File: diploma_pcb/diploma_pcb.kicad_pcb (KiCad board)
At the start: 2 copper layers, 50 x 24 mm, 16 parts, among them Q1 2SC3356, Q3 2SC3356

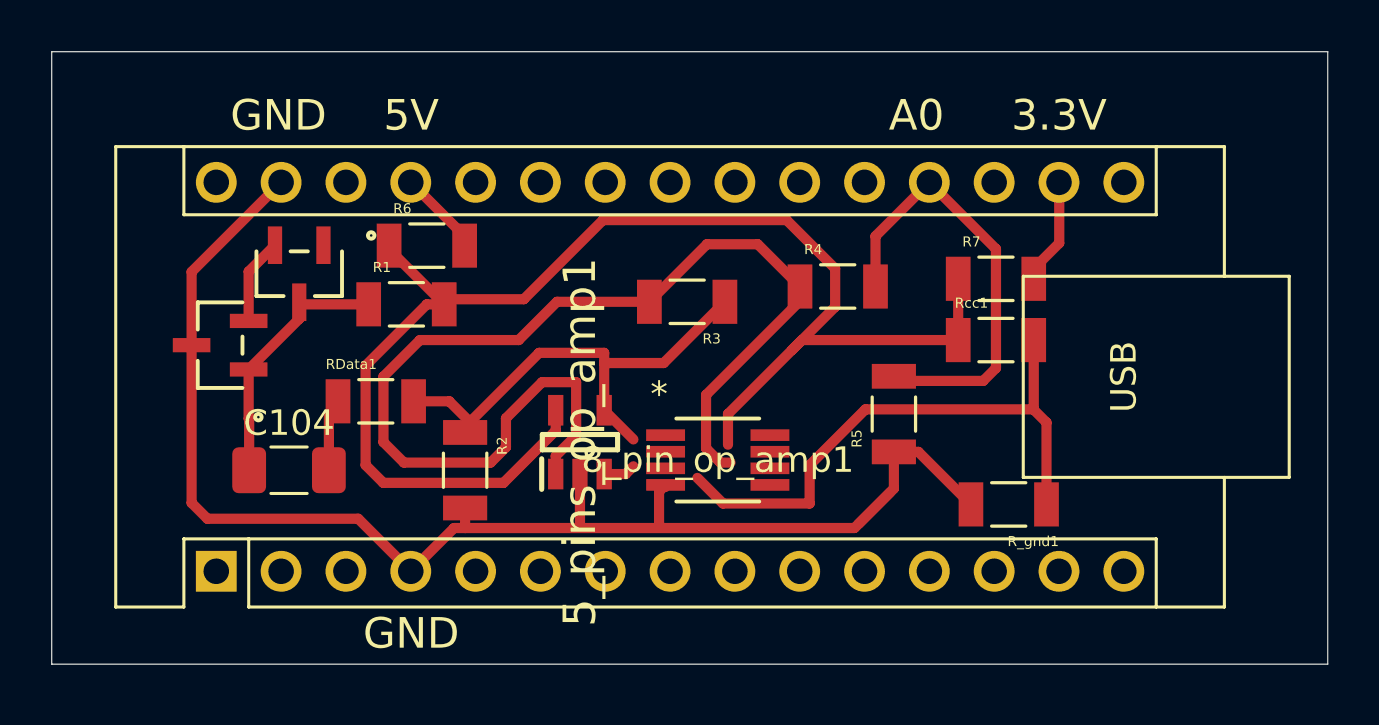
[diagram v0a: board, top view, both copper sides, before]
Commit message: with capacitors
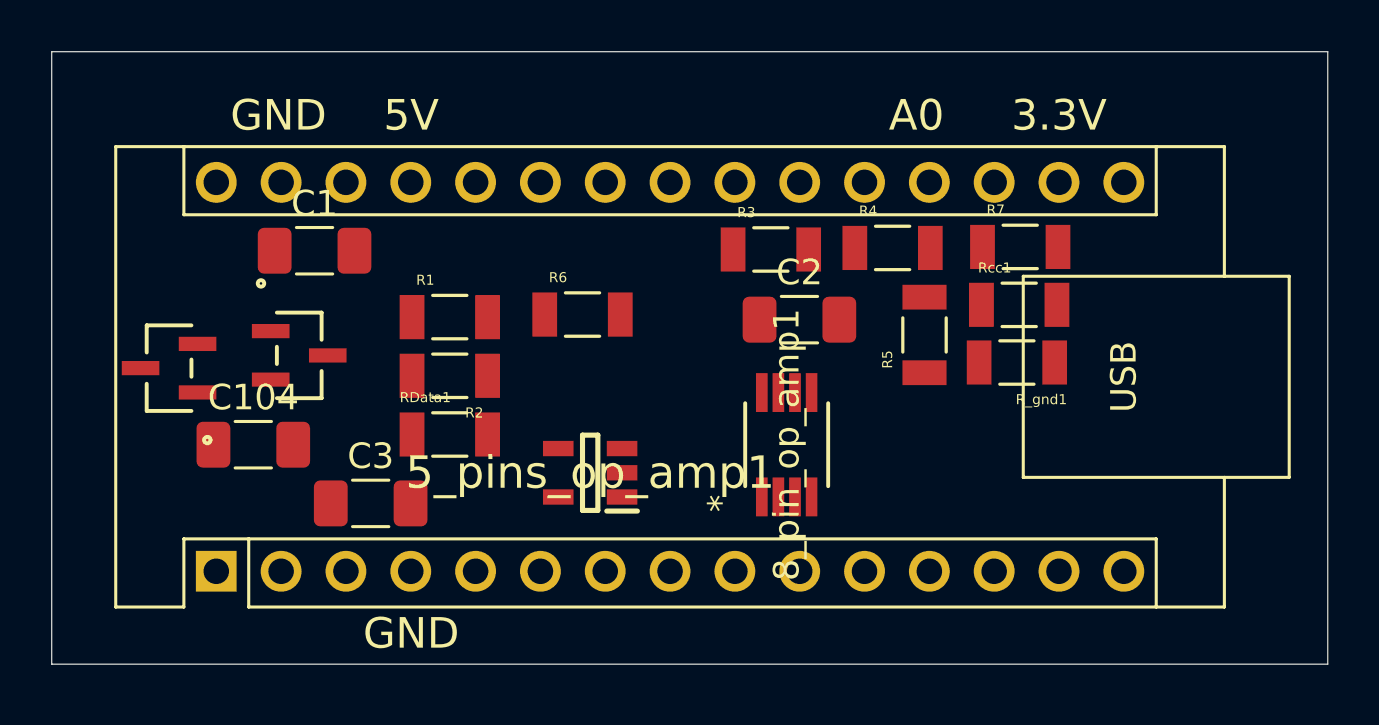
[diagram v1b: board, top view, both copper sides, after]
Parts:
- added C1: .1uF, Capacitor_SMD:C_1206_3216Metric_Pad1.33x1.80mm_HandSolder, F.Cu at (36.3, 57.3)
- added C2: .1uF, Capacitor_SMD:C_1206_3216Metric_Pad1.33x1.80mm_HandSolder, F.Cu at (55.3, 60.0)
- added C3: .1uF, Capacitor_SMD:C_1206_3216Metric_Pad1.33x1.80mm_HandSolder, F.Cu at (38.5, 67.2)
- moved R6 6.67 mm to (46.8, 59.8)
- moved R_gnd1 5.57 mm to (63.8, 61.7)
- moved R3 3.87 mm to (54.2, 57.2), turned to 0 degrees
- moved R2 3.75 mm to (41.6, 62.2), turned to 180 degrees
- moved R5 3.32 mm to (60.2, 60.6)
- moved Q1 3.20 mm to (35.7, 61.4), turned to -90 degrees
- moved RData1 3.18 mm to (41.6, 64.5)
- moved 8_pin_op_amp1 2.77 mm to (54.8, 64.9), turned to 90 degrees
- moved R4 2.63 mm to (59.0, 57.2)
- moved Q3 2.19 mm to (30.6, 61.9)
- moved R1 1.77 mm to (41.6, 59.9)
- moved C104 1.72 mm to (33.9, 64.9)
- moved Rcc1 1.65 mm to (63.9, 59.4)
- moved R7 1.57 mm to (64.0, 57.1)
- moved 5_pins_op_amp1 1.26 mm to (47.1, 66.0), turned to 180 degrees
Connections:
- 8_pin_op_amp1 pad 7: Net-(5_pins_op_amp1-VDD) -> Net-(8_pin_op_amp1-V+)
- R1 pad 2: Net-(5_pins_op_amp1-VDD) -> Net-(C1-Pad2)
- R6 pad 1: Net-(5_pins_op_amp1-VDD) -> Net-(C1-Pad2)
- R7 pad 1: Net-(5_pins_op_amp1-VDD) -> Net-(C1-Pad2)
- Rcc1 pad 1: Net-(5_pins_op_amp1-VDD) -> Net-(C1-Pad2)
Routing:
- net Net-(5_pins_op_amp1-VSS): track 56.1 -> 0.00 mm
- net Net-(5_pins_op_amp1-VDD): track 55.8 -> 0.00 mm
- net Net-(5_pins_op_amp1-VOUT): track 44.6 -> 0.00 mm
- net Net-(5_pins_op_amp1-VIN+): track 23.9 -> 0.00 mm
- net Net-(5_pins_op_amp1-VIN-): track 19.6 -> 0.00 mm
- net Net-(A1-A0): track 17.6 -> 0.00 mm
- net Net-(Q1-C): track 10.7 -> 0.00 mm
- net Net-(A1-3V3): track 4.20 -> 0.00 mm
- net Net-(Q1-B): track 3.40 -> 0.00 mm
- net Net-(A1-+5V): track 3.35 -> 0.00 mm
- net Net-(C104-Pad2): track 2.89 -> 0.00 mm
